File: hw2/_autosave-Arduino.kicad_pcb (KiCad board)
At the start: 2 copper layers, 28 parts, among them P1 CONN_01X02, P2 CONN_01X12, P3 CONN_01X12, P4 USB-A-PCB, U1 MIC5219, U2 ATmega32U4

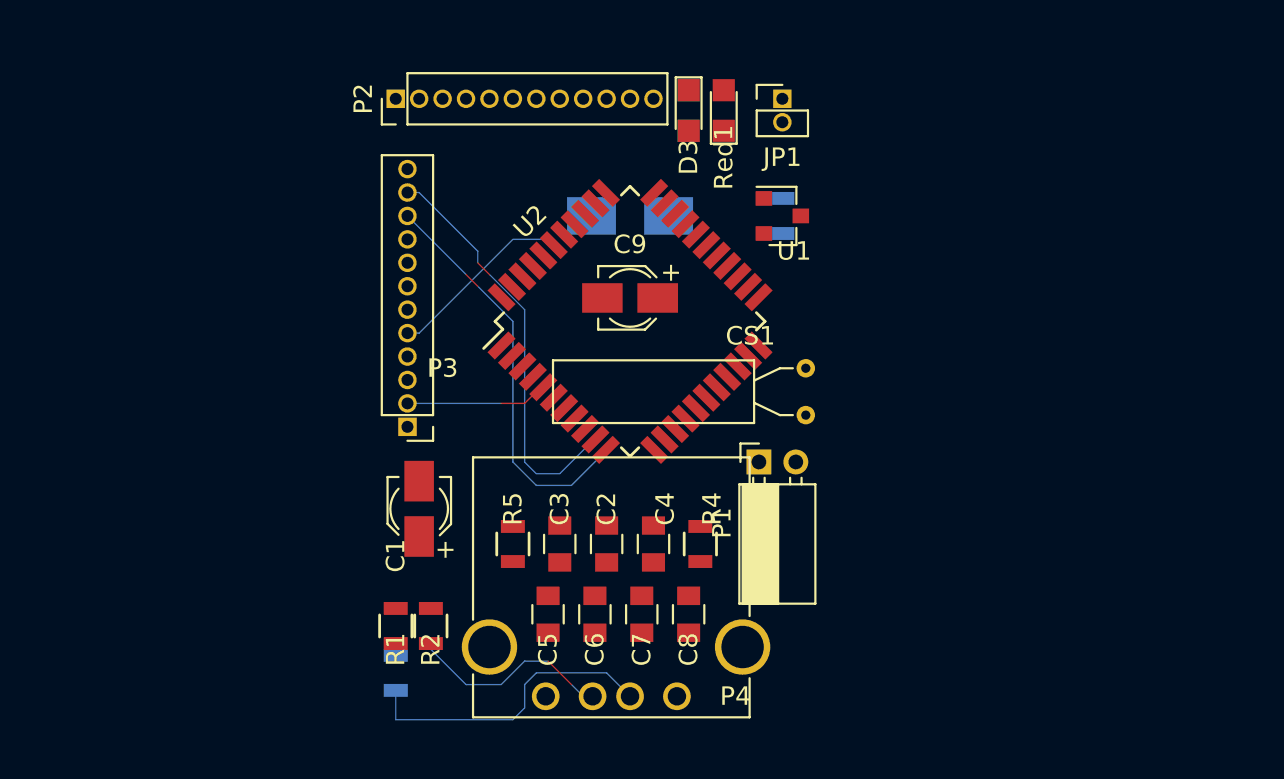
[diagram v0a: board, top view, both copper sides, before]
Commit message: Initial changes
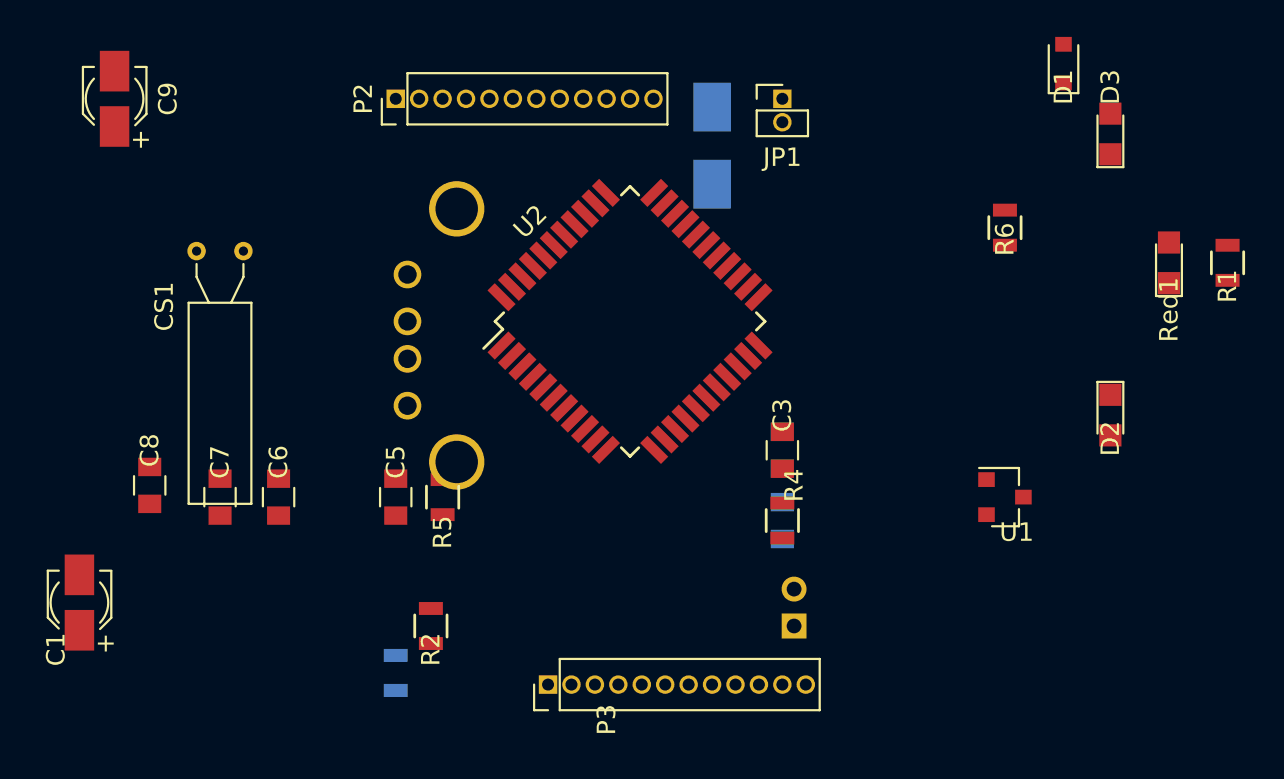
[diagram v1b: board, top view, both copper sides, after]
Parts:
- C2, C4, P1, P4: moved to B.Cu
- D1, D2, R6: moved to F.Cu
- moved R1 49.2 mm to (115.6, 52.7)
- moved CS1 33.6 mm to (59.7, 52.1), turned to 0 degrees
- moved C8 30.0 mm to (57.1, 64.8), turned to 270 degrees
- moved C9 30.0 mm to (55.2, 43.8), turned to 90 degrees
- moved D2 28.2 mm to (109.2, 61.0), turned to 270 degrees
- moved P4 27.1 mm to (71.1, 53.3), turned to 270 degrees
- moved Red1 25.5 mm to (112.4, 52.7)
- moved C7 23.7 mm to (61.0, 65.4), turned to 270 degrees
- moved D3 22.9 mm to (109.2, 45.7), turned to 90 degrees
- moved U1 19.4 mm to (103.5, 65.4)
- moved C1 19.1 mm to (53.3, 71.1)
- moved D1 18.6 mm to (106.7, 41.9), turned to 90 degrees
- moved C6 18.3 mm to (64.1, 65.4), turned to 270 degrees
- moved P3 15.9 mm to (78.7, 75.6), turned to 90 degrees
- moved C3 13.1 mm to (91.4, 62.9)
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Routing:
- net /MOSI: track 22.5 -> 0.00 mm, vias 2 -> 0
- net /MISO: track 22.1 -> 0.00 mm, vias 2 -> 0
- net Net-(P4-Pad2): track 16.6 -> 0.00 mm
- net Net-(P4-Pad3): track 10.9 -> 0.00 mm, vias 2 -> 0
- net /A3: track 9.72 -> 0.00 mm
- net GND: track 7.72 -> 0.00 mm, vias 1 -> 0
